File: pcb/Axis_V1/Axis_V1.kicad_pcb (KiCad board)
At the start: 2 copper layers, 114.3 x 63.5 mm, 38 parts, among them J1 TRANSDUCER, J11 3WAY_L, J2 Screw_Terminal_01x03, J3 BREW_SW, J4 STEAM_SW, J5 AC_L, J6 AC_N, J7 BOILER_SSR, J8 Screw_Terminal_01x02, J9 PUMP_L, Q1 BC547, Q2 BT136S-600, Q3 BT136S-600, U1 Pico, U2 ADS1115IDGS, U3 MAX31855KASA

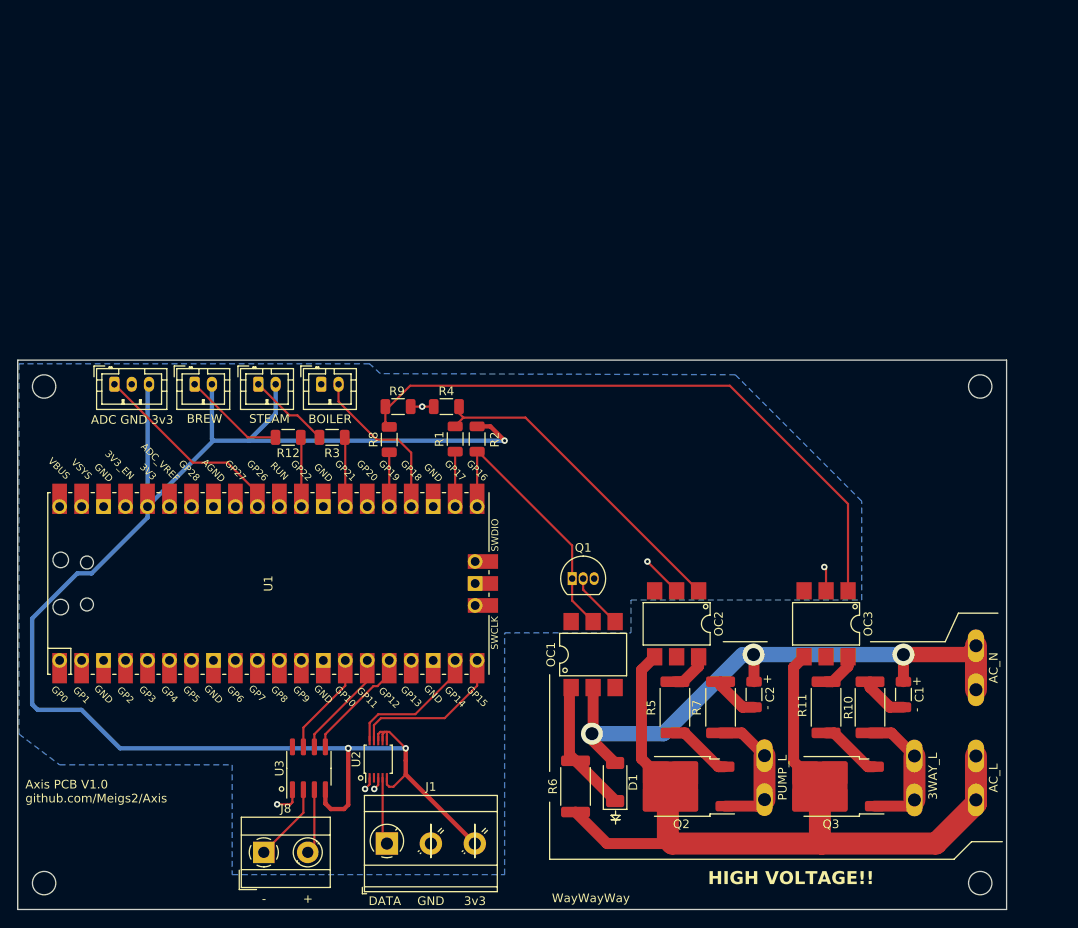
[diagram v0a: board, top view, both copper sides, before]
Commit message: Updates
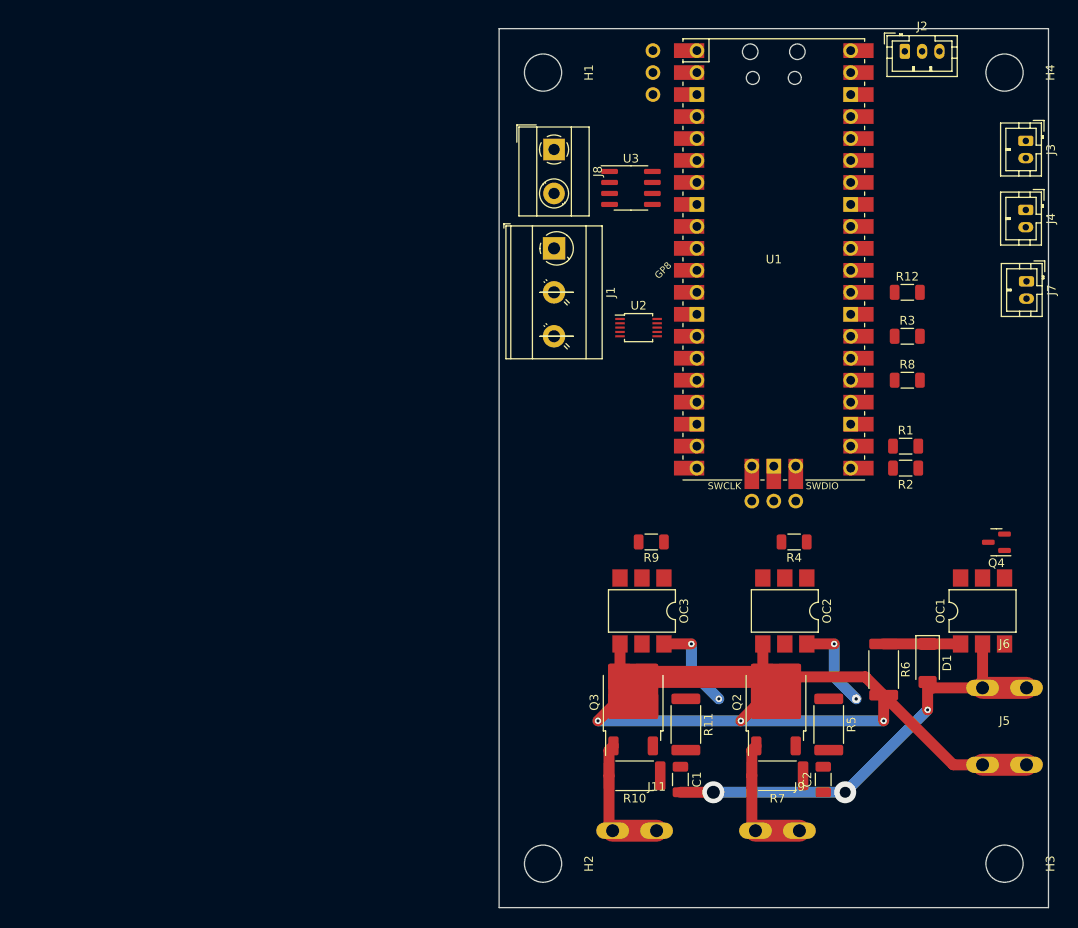
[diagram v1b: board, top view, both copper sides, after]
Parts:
- removed Q1: BC547, Package_TO_SOT_THT:TO-92_Inline
- added J10: Conn_01x03, Library:1x03 Pin Header Holes, F.Cu at (163.8, 30.5)
- added J12: Conn_01x03, Library:1x03 Pin Header Holes, F.Cu at (177.8, 80.0)
- added Q4: BC847, Package_TO_SOT_SMD:SOT-23, F.Cu at (203.5, 84.8)
- H1, H2, H3, H4: footprint MountingHole:MountingHole_2.7mm_M2.5 -> MountingHole:MountingHole_4.3mm_M4
- R6: value 470 -> 20k
- moved H1 110.0 mm to (151.1, 30.5), turned to -90 degrees
- moved J3 100.1 mm to (206.9, 38.4), turned to -90 degrees
- moved J2 99.1 mm to (192.9, 28.0)
- moved H4 93.7 mm to (204.5, 30.5), turned to -90 degrees
- moved J4 91.0 mm to (206.9, 46.4), turned to -90 degrees
- moved J8 87.9 mm to (152.4, 39.4), turned to -90 degrees
- moved J7 82.4 mm to (207.0, 54.6), turned to -90 degrees
- moved H2 79.8 mm to (151.1, 121.9), turned to -90 degrees
- moved U3 76.7 mm to (161.3, 43.8), turned to 0 degrees
- moved R12 73.5 mm to (193.2, 55.9), turned to 0 degrees
- moved J1 71.5 mm to (152.4, 50.8), turned to -90 degrees
- moved U1 69.4 mm to (177.8, 52.1), turned to 0 degrees
- moved R3 67.5 mm to (193.2, 61.0), turned to 0 degrees
- moved R8 60.3 mm to (193.2, 66.0), turned to 0 degrees
- moved U2 58.3 mm to (162.2, 60.0), turned to 0 degrees
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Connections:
- U1 pad 1: unconnected-(U1-GPIO0-Pad1) -> /UART_TX
- U1 pad 2: unconnected-(U1-GPIO1-Pad2) -> /UART_RX
- U1 pad 41: unconnected-(U1-SWCLK-Pad41) -> /SWCLK
- U1 pad 42: unconnected-(U1-GND-Pad42) -> GND
- U1 pad 43: unconnected-(U1-SWDIO-Pad43) -> /SWDIO
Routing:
- net +3.3V: track 187.7 -> 0.00 mm, vias 3 -> 0
- net Net-(OC3-Pad1): track 72.3 -> 0.00 mm
- net Net-(OC2-Pad1): track 38.3 -> 0.00 mm
- net /ZC_SIGNAL: track 31.8 -> 0.00 mm
- net /ADC_IN: track 24.9 -> 0.00 mm
- net /BOILER_GPIO: track 19.1 -> 0.00 mm
- net /ADS_SCL: track 18.5 -> 0.00 mm
- net /AC_N: track 69.9 -> 52.5 mm
- net GND: track 16.6 -> 0.00 mm, vias 6 -> 0
- net /ADS_SDA: track 15.9 -> 0.00 mm
- net /MAX_SCL: track 13.3 -> 0.00 mm
- net /MAX_CS: track 12.5 -> 0.00 mm
- net /MAX_SO: track 12.0 -> 0.00 mm
- net Net-(J3-Pin_1): track 11.9 -> 0.00 mm
- net Net-(J4-Pin_1): track 9.60 -> 0.00 mm
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- removed copper zone on B.Cu, net GND
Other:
- board size 114.3 x 63.5 mm -> 63.5 x 101.6 mm
- board text removed: "+"
- board text removed: "-"
- board text removed: "3v3"
- board text removed: "ADC GND 3v3"
- board text removed: "Axis PCB V1.0 github.com/Meigs2/Axis"
- board text removed: "BOILER"
- board text removed: "BREW"
- board text removed: "DATA"
- board text removed: "GND"
- board text removed: "HIGH VOLTAGE!!"
- board text removed: "STEAM"
- board text removed: "WayWayWay"
